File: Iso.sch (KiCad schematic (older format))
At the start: 7 parts, among them U12 Si8421

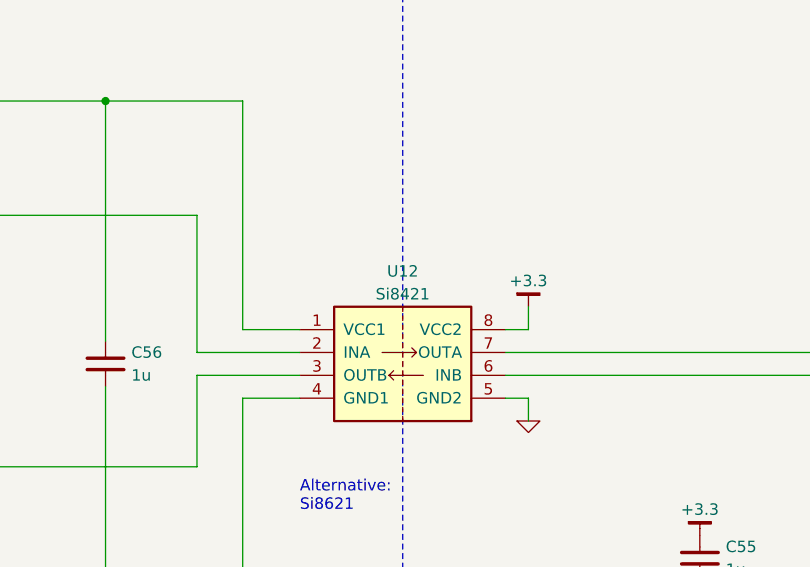
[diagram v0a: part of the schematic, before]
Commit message: Revise schematic
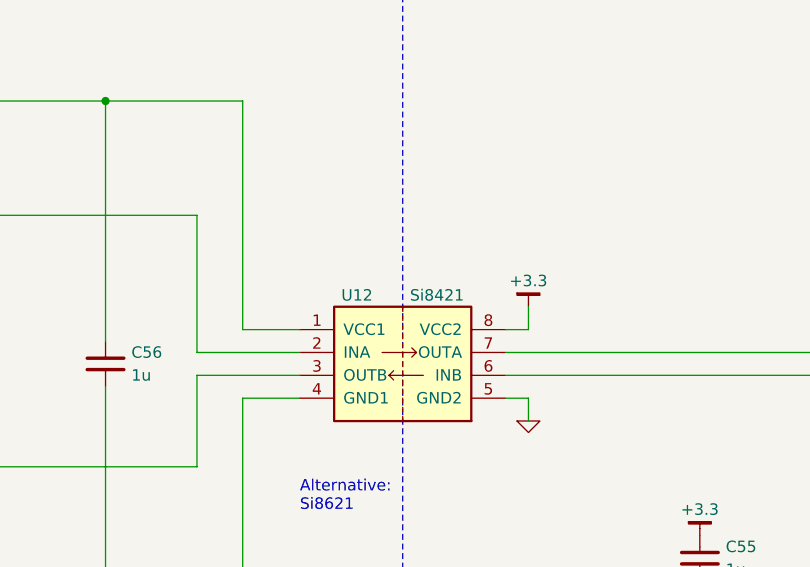
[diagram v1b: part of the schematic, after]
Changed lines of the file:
@@
 U 1 1 55D574BC
 P 6900 3750
-F 0 "U12" H 6900 4155 50  0000 C CNN
-F 1 "Si8421" H 6900 4055 50  0000 C CNN
+F 0 "U12" H 6700 4050 50  0000 C CNN
+F 1 "Si8421" H 7050 4050 50  0000 C CNN
 F 2 "IPC7351-Nominal:SOIC127P600X175-8" H 6900 3750 50  0001 C CNN
 F 3 "" H 6900 3750 60  0000 C CNN
